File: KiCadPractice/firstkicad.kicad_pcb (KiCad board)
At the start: 2 copper layers, 207 x 115.5 mm, 12 parts, among them Q1 BC337, U1 LM358, U2 LM358

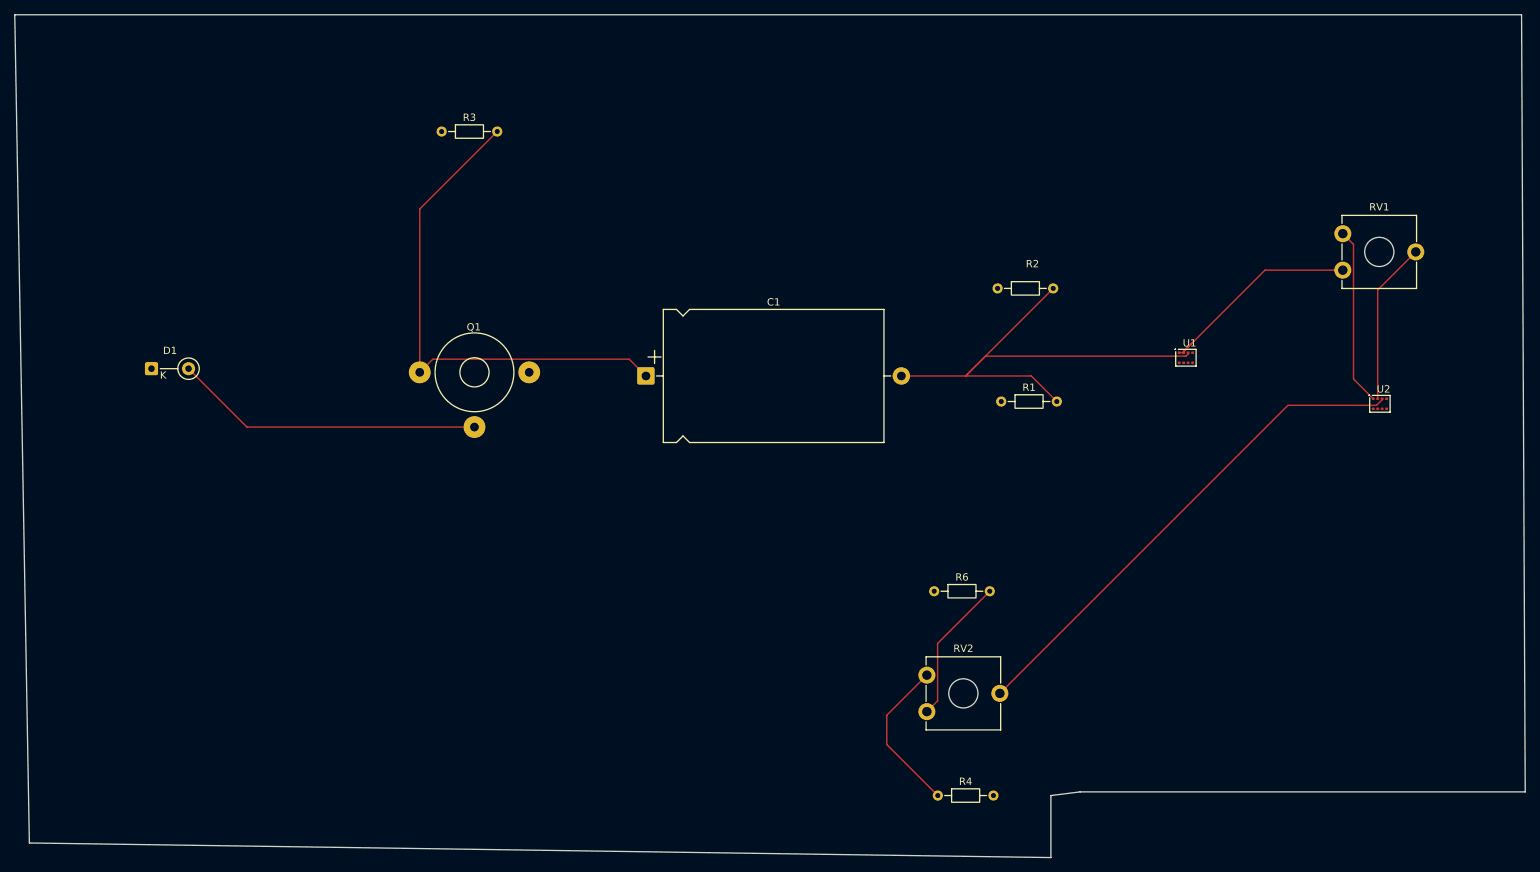
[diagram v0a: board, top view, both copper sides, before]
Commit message: Fixed edge-cuts.
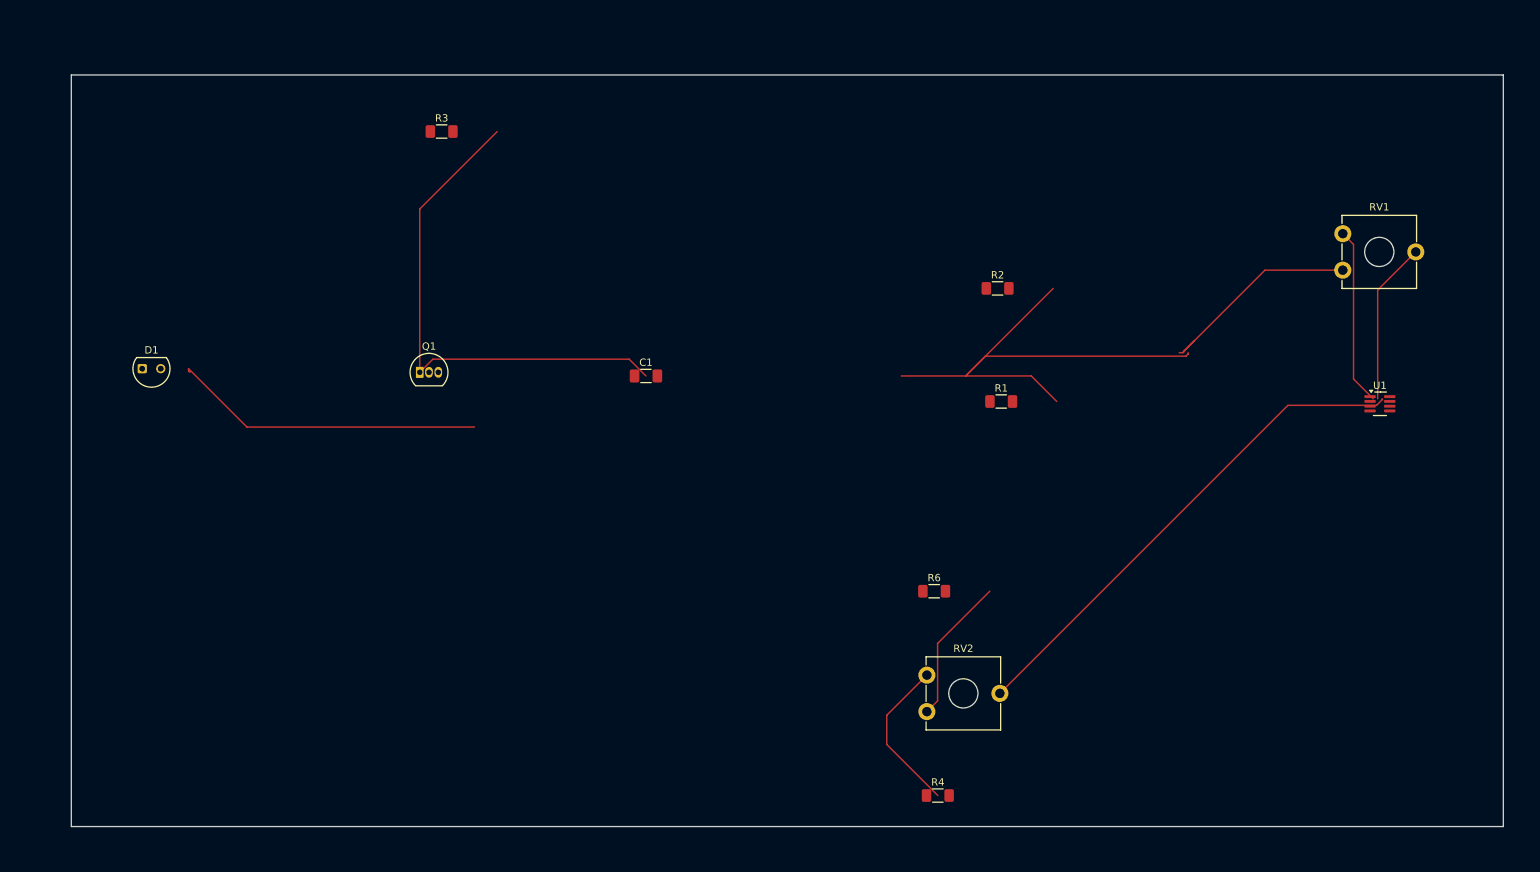
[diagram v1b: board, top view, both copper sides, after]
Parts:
- removed the U1 at (191.5, 99.5)
- C1: footprint Capacitor_THT:CP_Axial_L30.0mm_D18.0mm_P35.00mm_Horizontal -> Capacitor_SMD:C_1206_3216Metric_Pad1.33x1.80mm_HandSolder
- D1: value D_Photo -> LTR-516AD; footprint Diode_THT:D_A-405_P5.08mm_Vertical_KathodeUp -> Library:LTR-516AD
- Q1: footprint Transformer_THT:Autotransformer_Toroid_1Tap_Horizontal_D10.5mm_Amidon-T37 -> Package_TO_SOT_THT:TO-92_Inline
- R1, R2, R3, R4, R6: footprint Resistor_THT:R_Axial_DIN0204_L3.6mm_D1.6mm_P7.62mm_Horizontal -> Resistor_SMD:R_1206_3216Metric_Pad1.30x1.75mm_HandSolder
- U1: renamed from U2; footprint OptoDevice:Broadcom_APDS-9160-003 -> Package_TO_SOT_SMD:SOT-23-8_Handsoldering
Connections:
- D1 pad 1: 5 -> +5V
- R2 pad 1: 5 -> +5V
- R3 pad 1: 5 -> +5V
- R6 pad 1: 5 -> +5V
- RV1 pad 2: Net-(U2A--) -> Net-(U1B--)
- RV2 pad 2: Net-(U2A-+) -> Net-(U1B-+)
- U1 pad 1: Net-(RV1-Pad3) -> Net-(U1A--)
- U1 pad 2: Net-(U2A--) -> Net-(U1A--)
- U1 pad 3: Net-(U2A-+) -> Net-(U1A-+)
- U1 pad 4: (no net) -> +5V
- U1 pad 5: (no net) -> Net-(U1B-+)
- U1 pad 6: (no net) -> Net-(U1B--)
- U1 pad 7: (no net) -> Net-(RV1-Pad3)
- U1 pad 8: (no net) -> GND
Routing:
- net Net-(U1A--): track 29.4 -> 101.0 mm
- net Net-(U1A-+): track 71.6 -> 0.00 mm
- net Net-(U2A-+): track 69.2 -> 0.00 mm
- net (no net): track 0.00 -> 69.2 mm
- net Net-(U2A--): track 22.3 -> 0.00 mm
- net Net-(U1B--): track 0.00 -> 22.3 mm
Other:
- board size 207 x 115.5 mm -> 196.2 x 103 mm
